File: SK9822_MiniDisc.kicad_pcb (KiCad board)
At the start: 4 copper layers, 220 x 220 mm, 377 parts, among them P1 CONN_01X04, P2 CONN_01X04

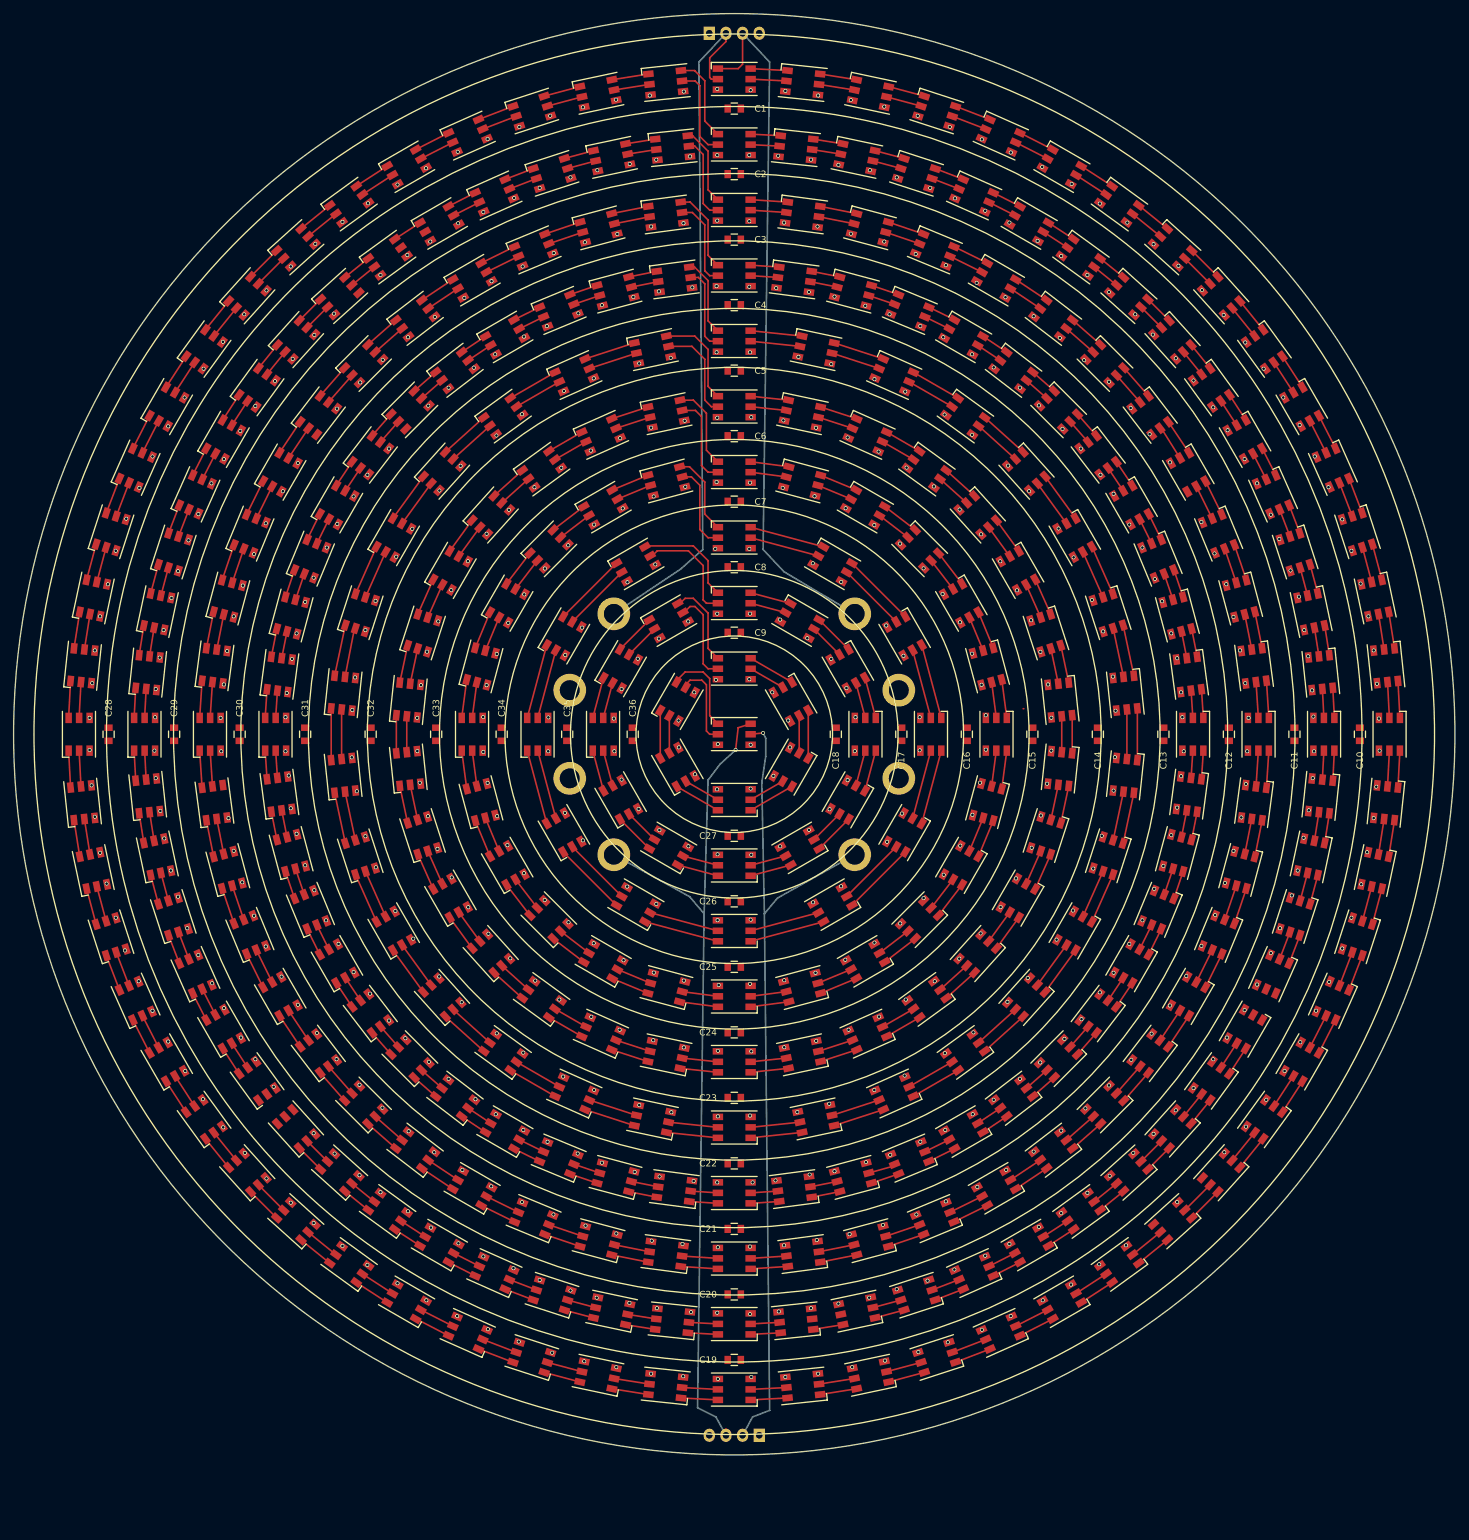
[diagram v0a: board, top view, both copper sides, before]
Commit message: finaly got caps right
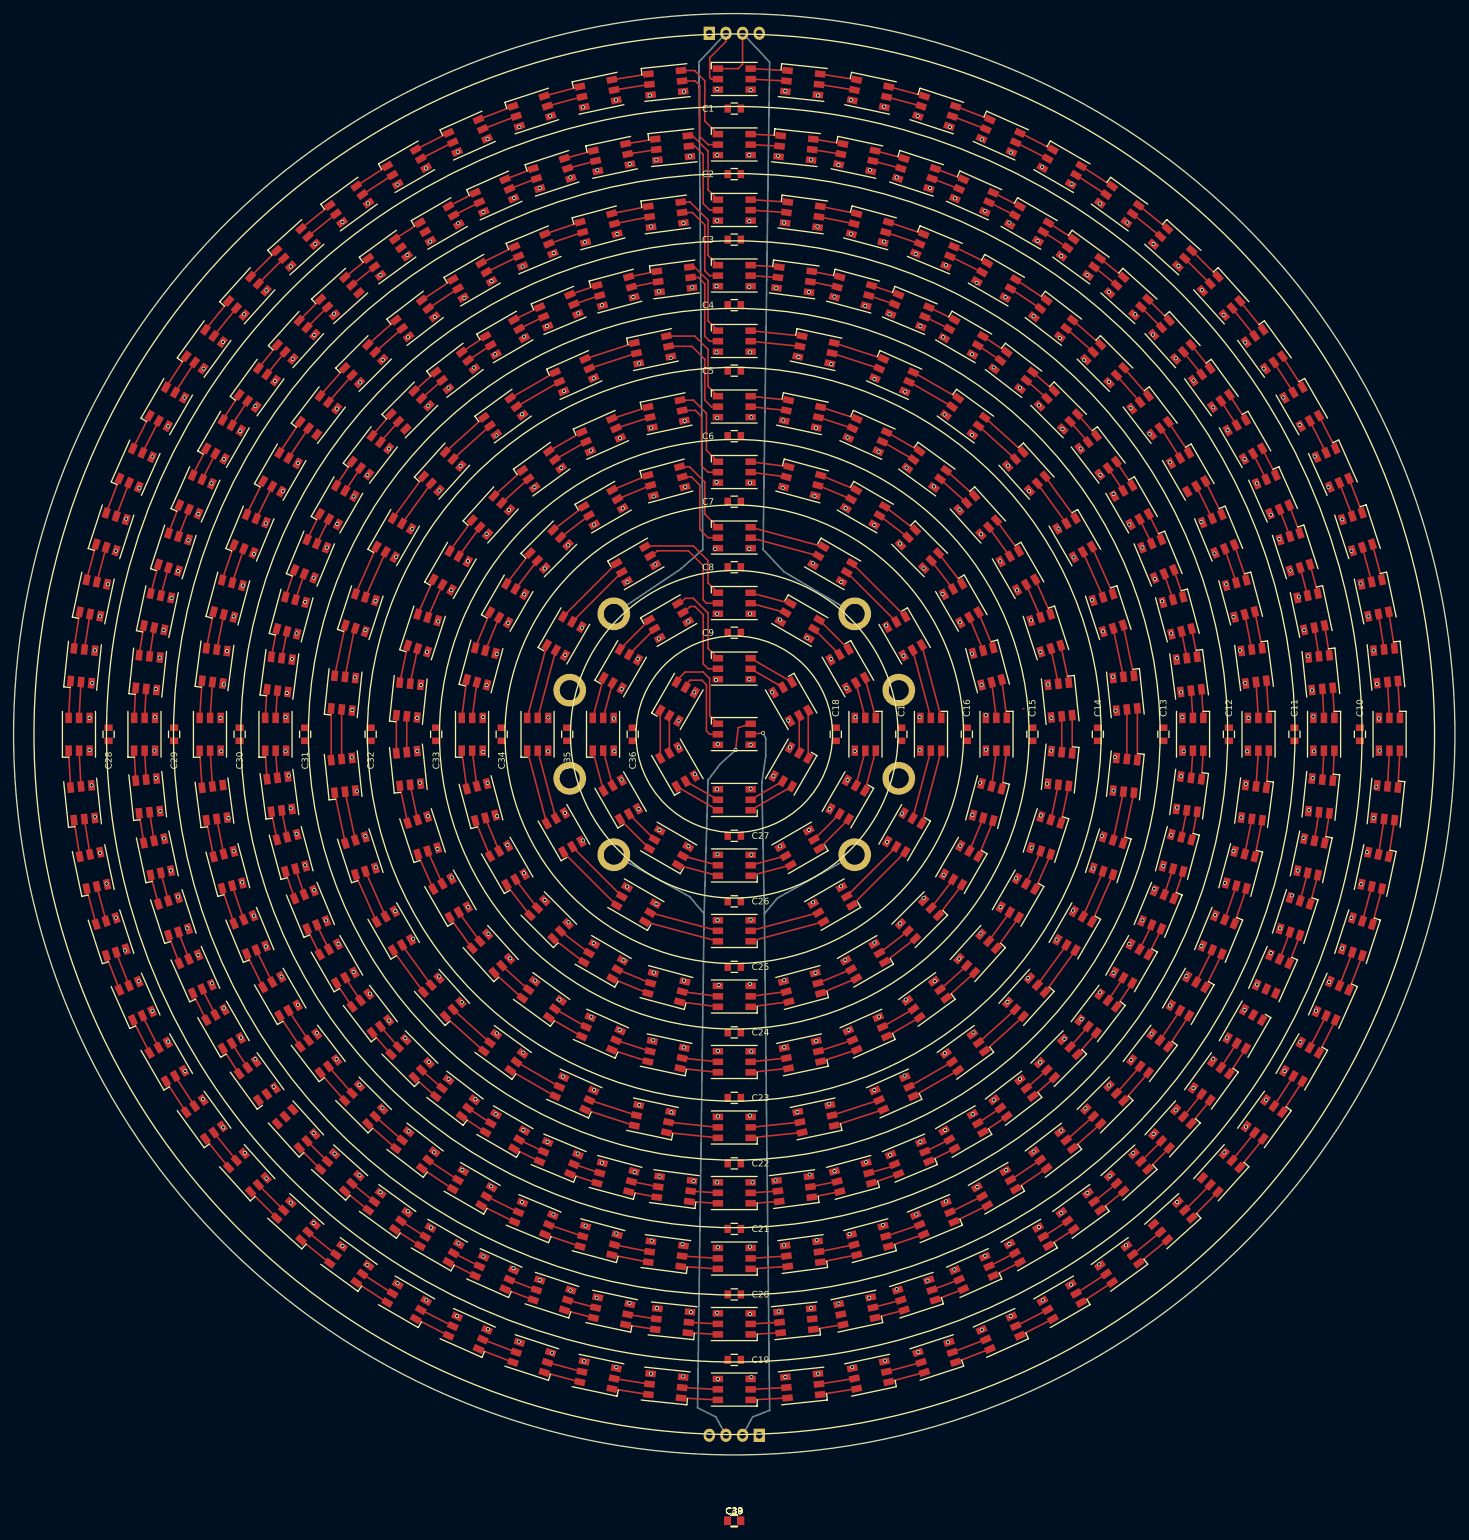
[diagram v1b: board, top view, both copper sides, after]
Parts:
- added C37, C38, C39, C40: 10uF, Capacitors_SMD:C_0805, F.Cu at (300.0, 320.1)
- C1, C10, C11, C12, C13, C14, C15, C16, C17, C18, C19, C2, C20, C21, C22, C23, C24, C25, C26, C27, C28, C29, C3, C30, C31, C32, C33, C34, C35, C36, C4, C5, C6, C7, C8, C9: value C_0805 -> 10uF
- turned C1 to 180 degrees
- turned C10 to 90 degrees
- turned C11 to 90 degrees
- turned C12 to 90 degrees
- turned C13 to 90 degrees
- turned C14 to 90 degrees
- turned C15 to 90 degrees
- turned C16 to 90 degrees
- turned C17 to 90 degrees
- turned C18 to 90 degrees
- turned C19 to 0 degrees
- turned C2 to 180 degrees
- turned C20 to 0 degrees
- turned C21 to 0 degrees
- turned C22 to 0 degrees
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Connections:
- C1 pad 1: (no net) -> VCC
- C1 pad 2: (no net) -> GND
- C10 pad 1: (no net) -> VCC
- C10 pad 2: (no net) -> GND
- C11 pad 1: (no net) -> VCC
- C11 pad 2: (no net) -> GND
- C12 pad 1: (no net) -> VCC
- C12 pad 2: (no net) -> GND
- C13 pad 1: (no net) -> VCC
- C13 pad 2: (no net) -> GND
- C14 pad 1: (no net) -> VCC
- C14 pad 2: (no net) -> GND
- C15 pad 1: (no net) -> VCC
- C15 pad 2: (no net) -> GND
- C16 pad 1: (no net) -> VCC
- C16 pad 2: (no net) -> GND
- C17 pad 1: (no net) -> VCC
- C17 pad 2: (no net) -> GND
- C18 pad 1: (no net) -> VCC
- C18 pad 2: (no net) -> GND
- C19 pad 1: (no net) -> VCC
- C19 pad 2: (no net) -> GND
- C2 pad 1: (no net) -> VCC
- C2 pad 2: (no net) -> GND
- C20 pad 1: (no net) -> VCC
- C20 pad 2: (no net) -> GND
- C21 pad 1: (no net) -> VCC
- C21 pad 2: (no net) -> GND
- C22 pad 1: (no net) -> VCC
- C22 pad 2: (no net) -> GND
- C23 pad 1: (no net) -> VCC
- C23 pad 2: (no net) -> GND
- C24 pad 1: (no net) -> VCC
- C24 pad 2: (no net) -> GND
- C25 pad 1: (no net) -> VCC
- C25 pad 2: (no net) -> GND
- C26 pad 1: (no net) -> VCC
- C26 pad 2: (no net) -> GND
- C27 pad 1: (no net) -> VCC
- C27 pad 2: (no net) -> GND
- C28 pad 1: (no net) -> VCC
- C28 pad 2: (no net) -> GND
- C29 pad 1: (no net) -> VCC
- C29 pad 2: (no net) -> GND
- C3 pad 1: (no net) -> VCC
- C3 pad 2: (no net) -> GND
- C30 pad 1: (no net) -> VCC
- C30 pad 2: (no net) -> GND
- C31 pad 1: (no net) -> VCC
- C31 pad 2: (no net) -> GND
- C32 pad 1: (no net) -> VCC
- C32 pad 2: (no net) -> GND
- C33 pad 1: (no net) -> VCC
- C33 pad 2: (no net) -> GND
- C34 pad 1: (no net) -> VCC
- C34 pad 2: (no net) -> GND
- C35 pad 1: (no net) -> VCC
- C35 pad 2: (no net) -> GND
- C36 pad 1: (no net) -> VCC
- C36 pad 2: (no net) -> GND
- C4 pad 1: (no net) -> VCC
- C4 pad 2: (no net) -> GND
- C5 pad 1: (no net) -> VCC
- C5 pad 2: (no net) -> GND
- C6 pad 1: (no net) -> VCC
- C6 pad 2: (no net) -> GND
- C7 pad 1: (no net) -> VCC
- C7 pad 2: (no net) -> GND
- C8 pad 1: (no net) -> VCC
- C8 pad 2: (no net) -> GND
- C9 pad 1: (no net) -> VCC
- C9 pad 2: (no net) -> GND
